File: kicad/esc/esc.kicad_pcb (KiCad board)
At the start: 4 copper layers, 101.6 x 118.1 mm, 109 parts, among them J2 Motor, Q1 IRF540N, Q2 IRF540N, Q3 IRF540N, Q4 IRF540N, Q5 IRF540N, Q6 IRF540N, Q7 2N3904, U1 IR2110, U10 4N35, U11 4N35, U12 4N35, U13 4N35, U14 4N35, U15 4N35, U2 IR2110, U3 IR2110, U4 LM393, U5 LM393, U6 LM7805_TO220, U7 4N35, U8 4N35, U9 4N35

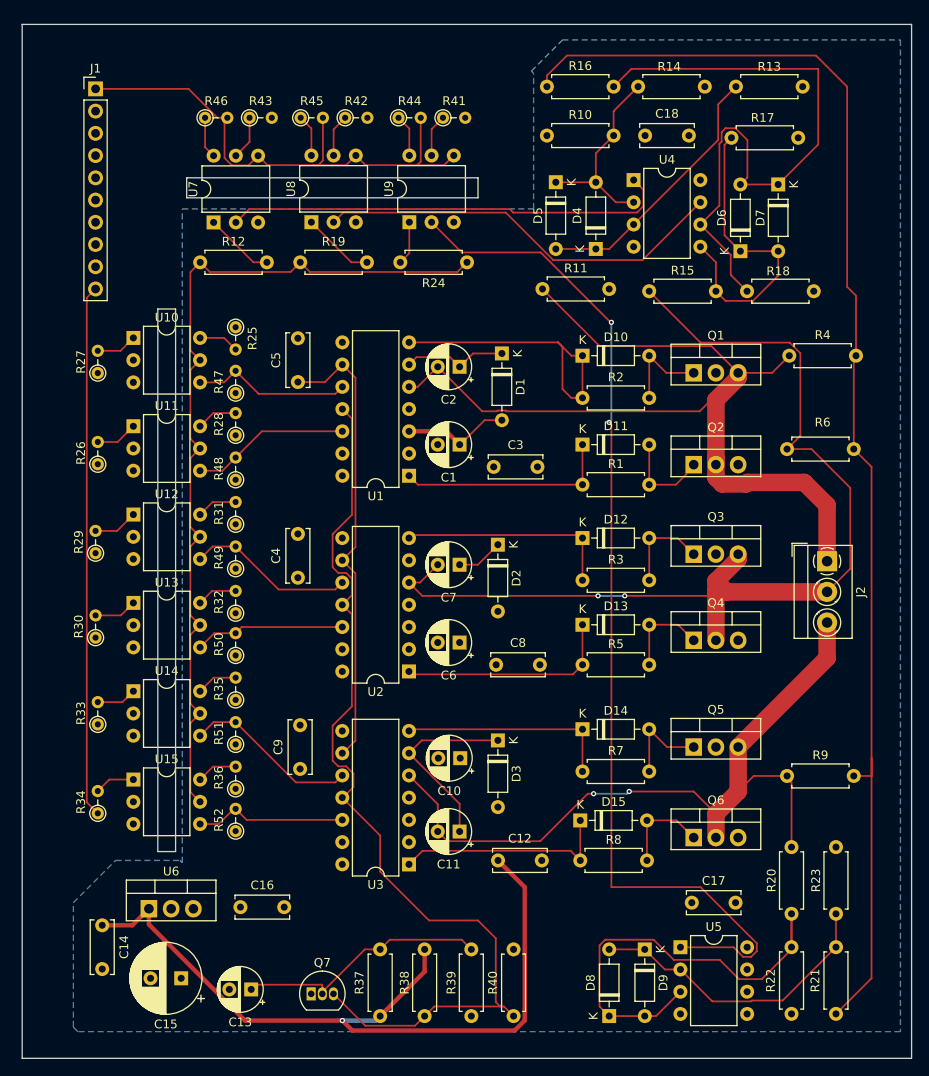
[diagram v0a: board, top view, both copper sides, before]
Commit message: WIP
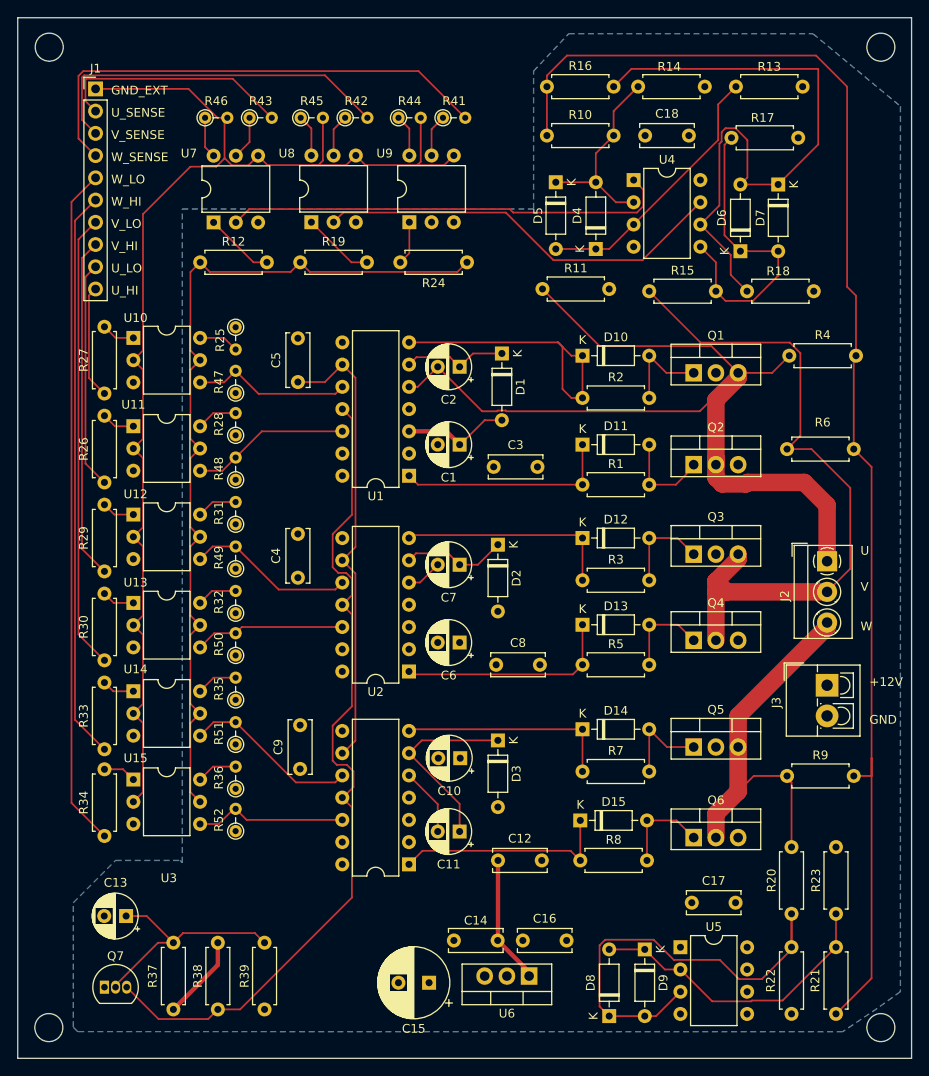
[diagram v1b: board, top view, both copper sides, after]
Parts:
- removed R40: 6.8k, Resistor_THT:R_Axial_DIN0207_L6.3mm_D2.5mm_P7.62mm_Horizontal
- added J3: Screw_Terminal_01x02, TerminalBlock_4Ucon:TerminalBlock_4Ucon_1x02_P3.50mm_Vertical, F.Cu at (117.9, 100.9)
- added REF**: MountingHole_3.2mm_M3, MountingHole:MountingHole_3.2mm_M3, F.Cu at (29.0, 140.0)
- added REF**: MountingHole_3.2mm_M3, MountingHole:MountingHole_3.2mm_M3, F.Cu at (124.0, 140.0)
- added REF**: MountingHole_3.2mm_M3, MountingHole:MountingHole_3.2mm_M3, F.Cu at (29.0, 28.0)
- added REF**: MountingHole_3.2mm_M3, MountingHole:MountingHole_3.2mm_M3, F.Cu at (124.0, 28.0)
- R26, R27, R29, R30, R33, R34: footprint Resistor_THT:R_Axial_DIN0204_L3.6mm_D1.6mm_P2.54mm_Vertical -> Resistor_THT:R_Axial_DIN0207_L6.3mm_D2.5mm_P7.62mm_Horizontal
- moved C14 45.2 mm to (80.2, 130.0), turned to 180 degrees
- moved U6 44.1 mm to (83.8, 134.1), turned to 180 degrees
- moved C16 32.5 mm to (83.1, 130.0)
- moved C15 28.3 mm to (72.4, 134.9)
- moved R37 23.6 mm to (43.2, 137.9)
- moved R38 23.6 mm to (48.3, 130.3)
- moved Q7 23.6 mm to (35.3, 135.4)
- moved R39 23.6 mm to (53.6, 130.3)
- moved C13 16.6 mm to (37.8, 127.3)
- moved R33 2.94 mm to (35.3, 108.2)
- moved R30 2.78 mm to (35.3, 98.0)
- moved R34 2.70 mm to (35.3, 118.1)
- moved R27 2.46 mm to (35.3, 67.6)
- moved R29 2.32 mm to (35.3, 87.9)
- moved R26 2.22 mm to (35.3, 77.7)
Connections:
- J1 pad 10: W_LO -> U_HI
- J1 pad 5: U_HI -> W_LO
- J1 pad 6: U_LO -> W_HI
- J1 pad 7: V_HI -> V_LO
- J1 pad 8: V_LO -> V_HI
- J1 pad 9: W_HI -> U_LO
- R37 pad 1: +12V -> +5V
- R38 pad 1: +12V -> +5V
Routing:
- net GND_EXT: track 61.7 -> 145.8 mm
- net +12V: track 102.5 -> 27.1 mm, vias 1 -> 0
- net W_HI: track 0.00 -> 65.1 mm
- net W_SENSE: track 0.00 -> 56.5 mm
- net V_LO: track 0.00 -> 52.1 mm
- net V_SENSE: track 0.00 -> 41.7 mm
- net V_HI: track 0.00 -> 39.0 mm
- net U_SENSE: track 0.00 -> 27.3 mm
- net U_LO: track 0.00 -> 26.0 mm
- net W_LO: track 60.8 -> 77.9 mm
- net Net-(U5-Pad1): track 119.6 -> 105.2 mm, vias 2 -> 0
- net Net-(Q7-C): track 109.2 -> 96.1 mm
- net U_HI: track 0.00 -> 13.0 mm
- net +5V: track 152.3 -> 162.0 mm
- net Net-(D2-K): track 5.32 -> 12.0 mm
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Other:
- board size 101.6 x 118.1 mm -> 102.1 x 118.9 mm
- board text added: "+12V"
- board text added: "GND"
- board text added: "GND_EXT"
- board text added: "U"
- board text added: "U_HI"
- board text added: "U_LO"
- board text added: "U_SENSE"
- board text added: "V"
- board text added: "V_HI"
- board text added: "V_LO"
- board text added: "V_SENSE"
- board text added: "W"
- board text added: "W_HI"
- board text added: "W_LO"
- board text added: "W_SENSE"
